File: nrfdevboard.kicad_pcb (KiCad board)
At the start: 4 copper layers, 56 x 88 mm, 15 parts, among them J1 USB2.0, J3 Conn_01x17_Pin, J4 Conn_01x17_Pin, U1 MDBT50Q-P1MV2, Y1 32.768

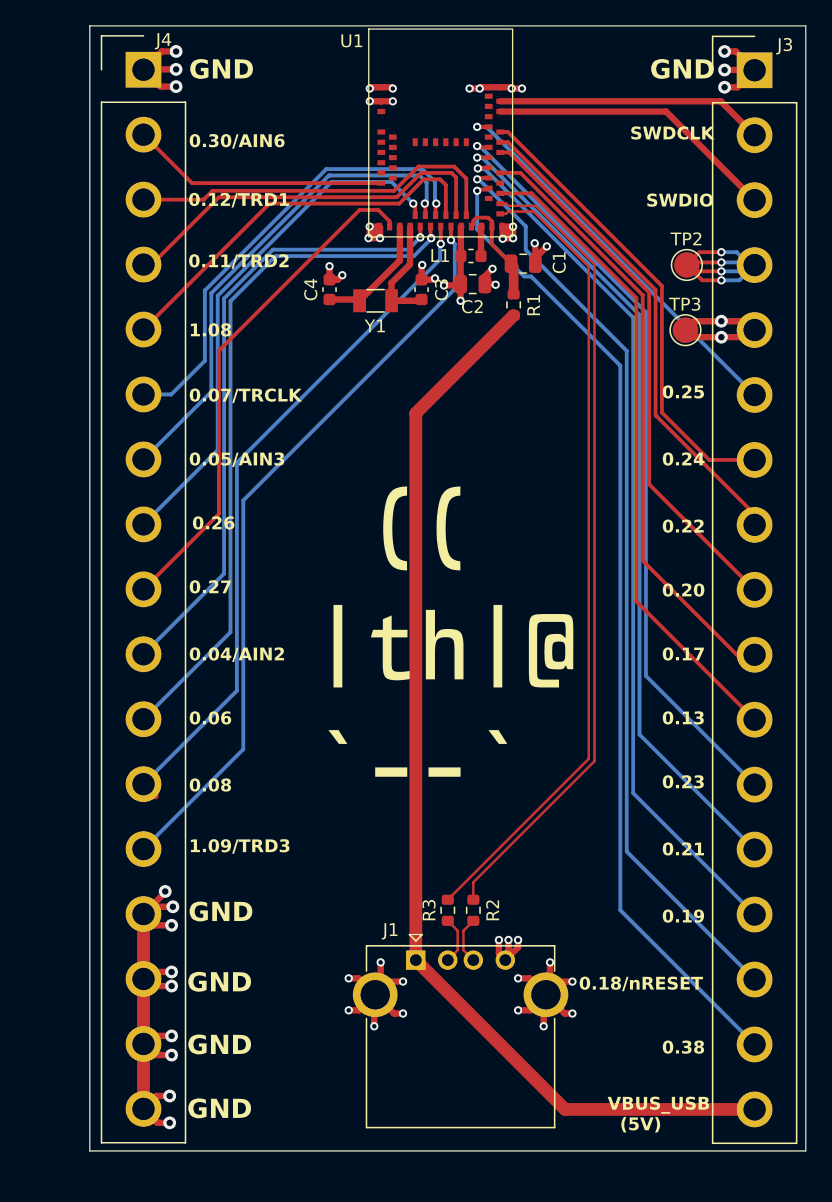
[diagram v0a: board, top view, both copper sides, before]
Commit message: Teardrops and grid origins.
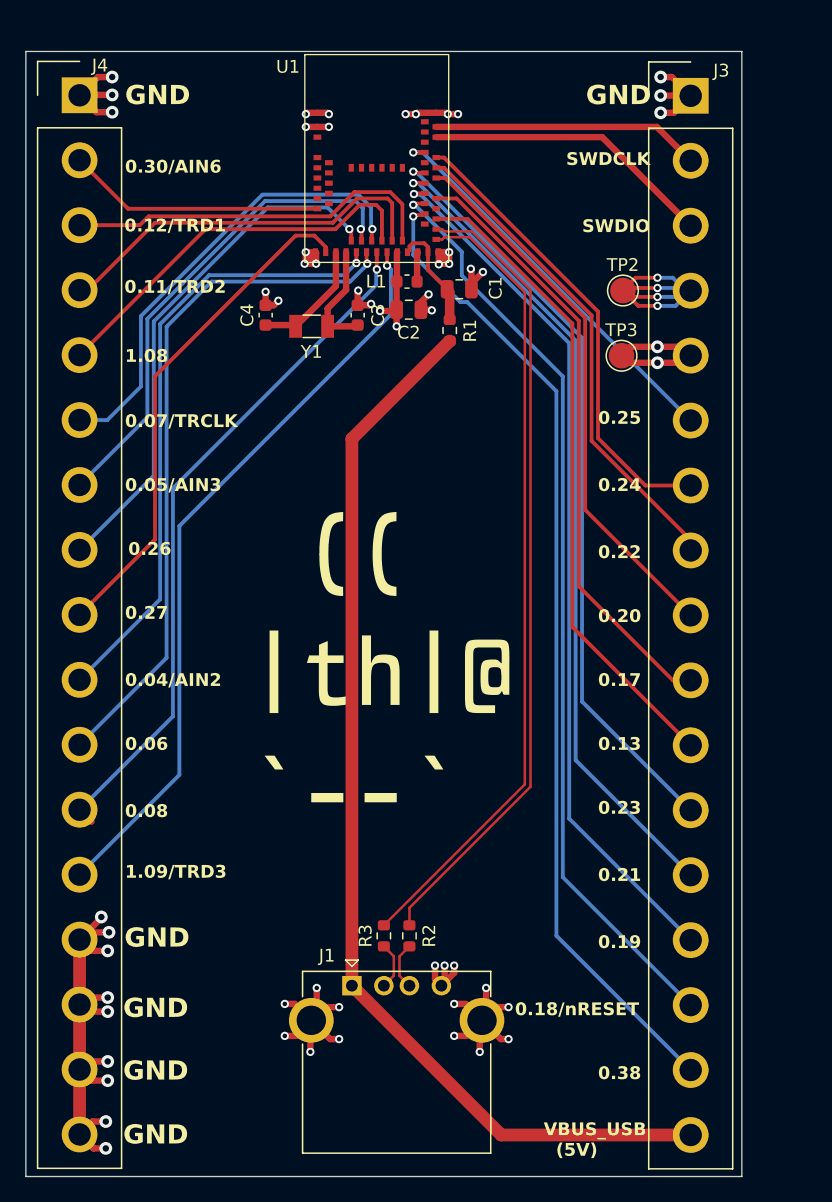
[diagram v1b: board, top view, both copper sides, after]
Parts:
- moved U1 5.39 mm to (101.7, 52.2)
- moved C1 5.39 mm to (113.9, 70.6)
- moved C2 5.39 mm to (110.0, 72.2)
- moved C3 5.39 mm to (106.0, 72.6)
- moved C4 5.39 mm to (98.8, 72.6)
- moved J1 5.39 mm to (105.5, 125.1)
- moved J3 5.39 mm to (132.0, 55.5)
- moved J4 5.39 mm to (84.2, 55.4)
- moved L1 5.39 mm to (109.8, 70.0)
- moved R1 5.39 mm to (113.2, 73.8)
- moved R2 5.39 mm to (110.0, 121.2)
- moved R3 5.39 mm to (108.0, 121.2)
- moved TP3 5.39 mm to (126.6, 75.8)
- moved Y1 5.39 mm to (102.4, 73.5)
- moved TP2 5.39 mm to (126.7, 70.7)
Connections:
- J1 pad 5: (no net) -> GND
